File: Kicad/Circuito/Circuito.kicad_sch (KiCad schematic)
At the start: 3 parts

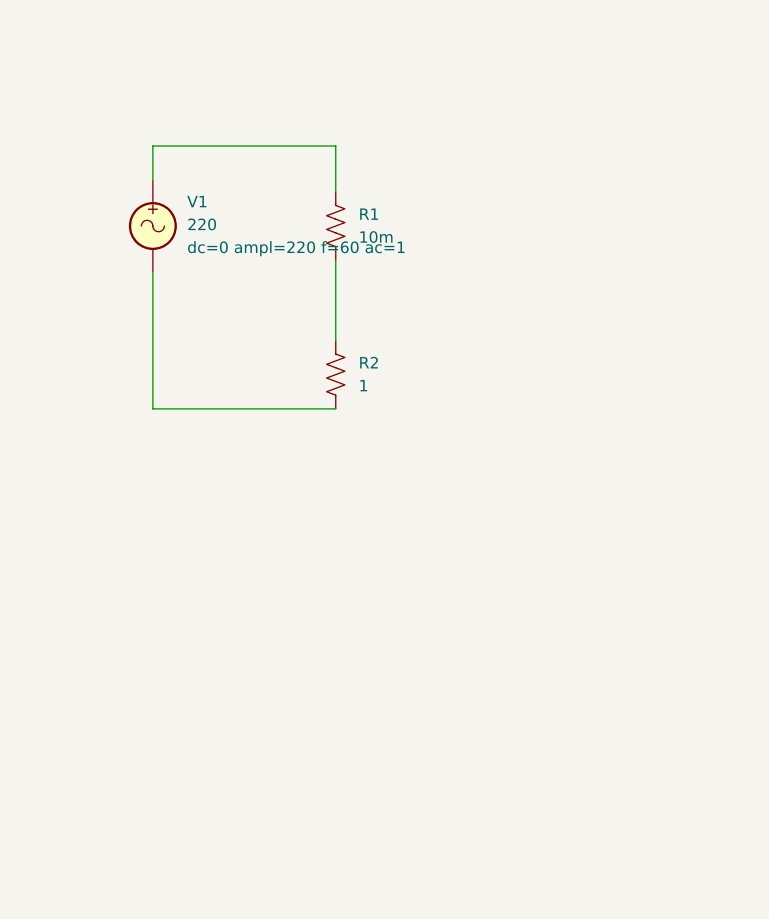
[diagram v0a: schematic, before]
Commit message: kicad
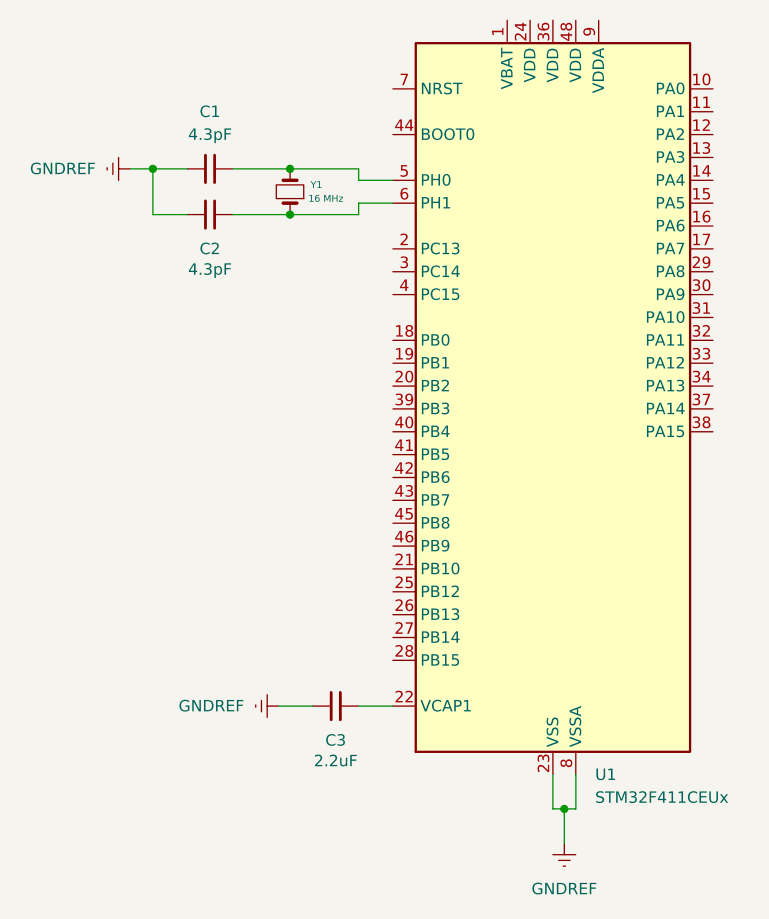
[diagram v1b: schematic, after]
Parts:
- removed R1: 10m, symbol Device:R_US
- removed R2: 1, symbol Device:R_US
- removed V1: 220, symbol Simulation_SPICE:VSIN
- added C1, C2: 4.3pF, symbol Device:C_Small
- added C3: 2.2uF, symbol Device:C_Small
- added U1: STM32F411CEUx, Package_DFN_QFN:QFN-48-1EP_7x7mm_P0.5mm_EP5.6x5.6mm, symbol MCU_ST_STM32F4:STM32F411CEUx
- added Y1: 16 MHz, Crystal:Crystal_HC49-U_Vertical, symbol Device:Crystal_Small
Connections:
- new net: C2.2, U1.6 (PH1), Y1.1
- new net: C1.2, U1.5 (PH0), Y1.2
- new net: C3.2, U1.22 (VCAP1)
- new net GNDREF: C1.1, C2.1, C3.1, U1.23 (VSS), U1.35 (VSS), U1.47 (VSS), U1.49 (VSS), U1.8 (VSSA)
